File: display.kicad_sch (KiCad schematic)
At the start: 3 parts, among them J14 LH397K

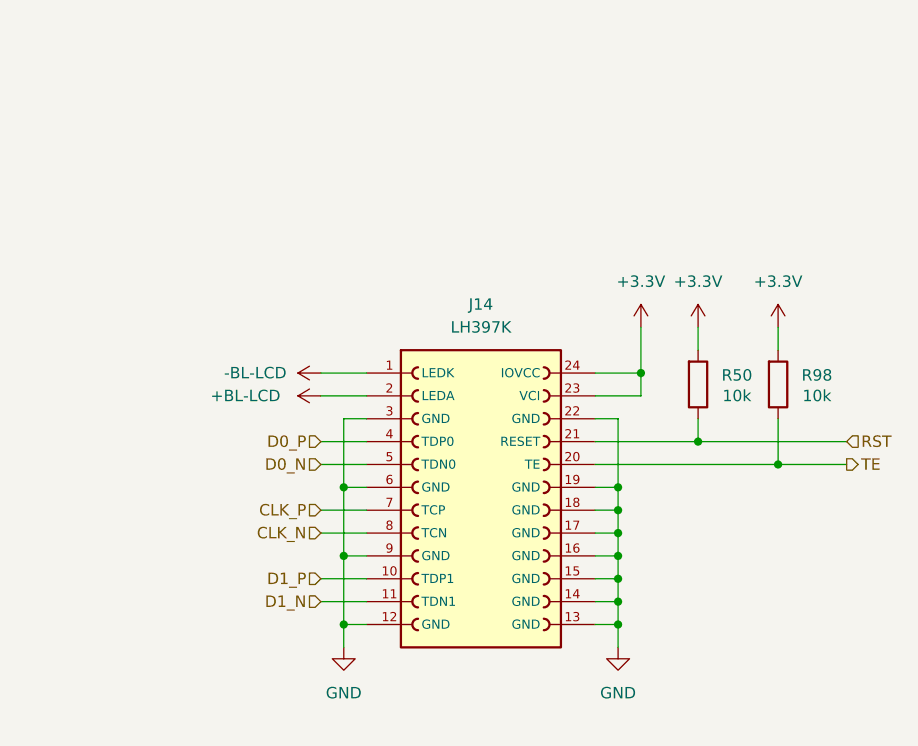
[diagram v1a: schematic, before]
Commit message: 18-Add correct display connector
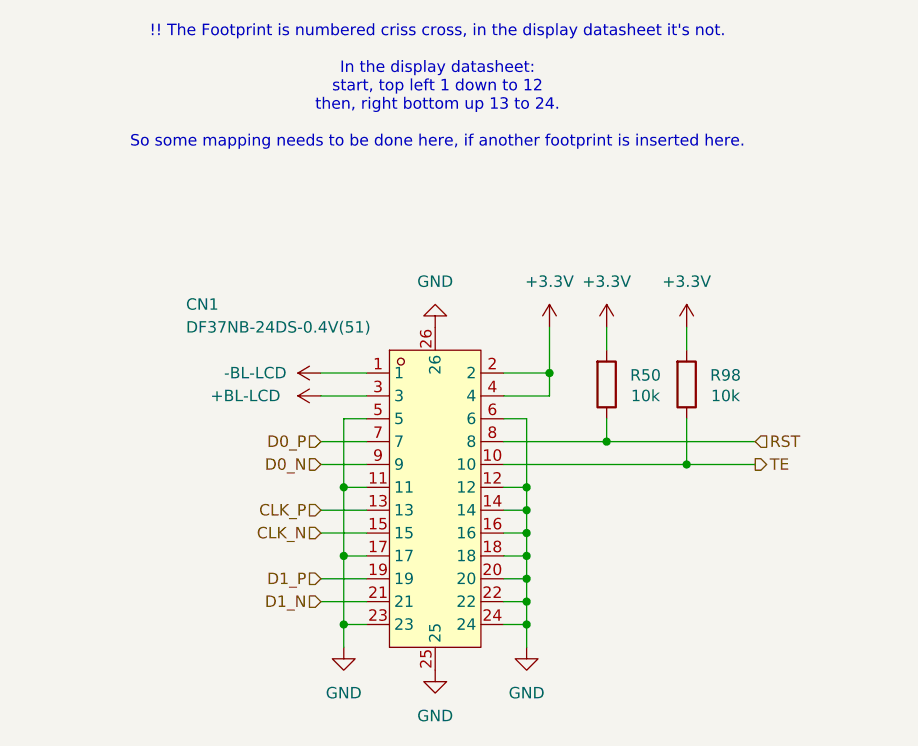
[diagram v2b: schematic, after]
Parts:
- removed J14: LH397K, library:LH397K-IC01, symbol LH397K-IC01:LH397K-IC01
- added CN1: DF37NB-24DS-0.4V(51), lcsc:CONN-SMD_DF37NB-24DS-0.4V, symbol lcsc:DF37NB-24DS-0.4V(51)
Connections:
- net +3.3V: now also CN1.2, CN1.4
- net +BL-LCD: now also CN1.3
- net -BL-LCD: now also CN1.1
- net CLK_N: now also CN1.15
- net CLK_P: now also CN1.13
- net D0_N: now also CN1.9
- net D0_P: now also CN1.7
- net D1_N: now also CN1.21
- net D1_P: now also CN1.19
- net GND: now also CN1.11, CN1.12, CN1.14, CN1.16, CN1.17, CN1.18, CN1.20, CN1.22, CN1.23, CN1.24, CN1.25, CN1.26, CN1.5, CN1.6
- net RST: now also CN1.8
- net TE: now also CN1.10
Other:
- note added: "!! The Footprint is numbered criss cross, in the display datasheet it's not. In the display datasheet: start, top left 1 down to 12 then, right bottom up 13 to 24. So some mapping needs to be done here, if another footprint is inserted here."
- moved on the sheet: R50, R98

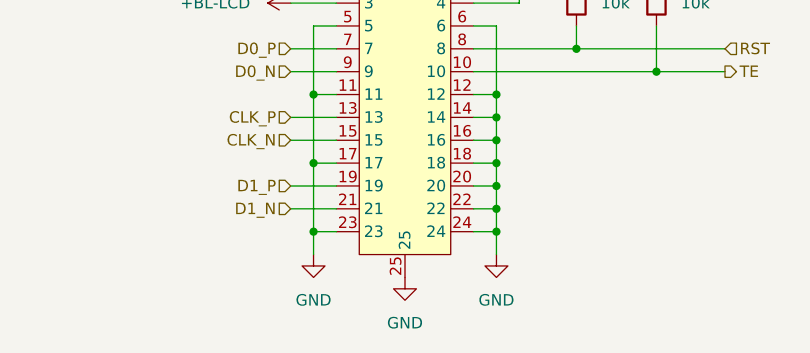
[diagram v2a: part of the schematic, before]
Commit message: Disconnect PG from reset of P4, connect to GPIO of CH32, fix warnings, make some vias bigger, add BHI360
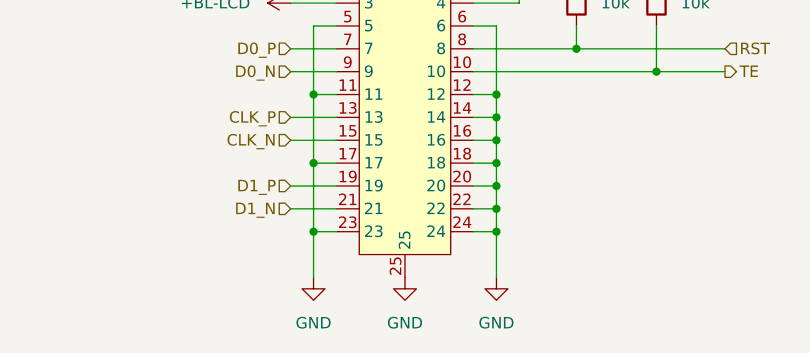
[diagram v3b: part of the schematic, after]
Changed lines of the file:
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@@
 	(wire
 		(pts
-			(xy 133.35 106.68) (xy 133.35 109.22)
+			(xy 133.35 106.68) (xy 133.35 111.76)
 		)
 		(stroke
@@
 	(wire
 		(pts
-			(xy 153.67 106.68) (xy 153.67 109.22)
+			(xy 153.67 106.68) (xy 153.67 111.76)
 		)
 		(stroke
@@
 	(symbol
 		(lib_id "power:GND")
-		(at 133.35 109.22 0)
+		(at 133.35 111.76 0)
 		(unit 1)
 		(exclude_from_sim no)
@@
 		(fields_autoplaced yes)
 		(property "Reference" "#PWR0190"
-			(at 133.35 115.57 0)
+			(at 133.35 118.11 0)
 			(effects
 				(font
@@
 		)
 		(property "Value" "GND"
-			(at 133.35 114.3 0)
+			(at 133.35 116.84 0)
 			(effects
 				(font
@@
 		)
 		(property "Footprint" ""
-			(at 133.35 109.22 0)
+			(at 133.35 111.76 0)
 			(effects
 				(font
@@
 		)
 		(property "Datasheet" ""
-			(at 133.35 109.22 0)
+			(at 133.35 111.76 0)
 			(effects
 				(font
@@
 		)
 		(property "Description" ""
-			(at 133.35 109.22 0)
+			(at 133.35 111.76 0)
 			(effects
 				(font
@@
 	(symbol
 		(lib_id "power:GND")
-		(at 153.67 109.22 0)
+		(at 153.67 111.76 0)
 		(unit 1)
 		(exclude_from_sim no)
@@
 		(fields_autoplaced yes)
 		(property "Reference" "#PWR0191"
-			(at 153.67 115.57 0)
+			(at 153.67 118.11 0)
 			(effects
 				(font
@@
 		)
 		(property "Value" "GND"
-			(at 153.67 114.3 0)
+			(at 153.67 116.84 0)
 			(effects
 				(font
@@
 		)
 		(property "Footprint" ""
-			(at 153.67 109.22 0)
+			(at 153.67 111.76 0)
 			(effects
 				(font
@@
 		)
 		(property "Datasheet" ""
-			(at 153.67 109.22 0)
+			(at 153.67 111.76 0)
 			(effects
 				(font
@@
 		)
 		(property "Description" ""
-			(at 153.67 109.22 0)
-			(effects
-				(font
+			(at 153.67 111.76 0)
+			(effects
+				(font
